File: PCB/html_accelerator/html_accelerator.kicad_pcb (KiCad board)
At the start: 4 copper layers, 129.3 x 104.4 mm, 170 parts, among them J1 Bus_PCI_Express_x16, J2 PCIexpress_bracket, U1 MCS9990, U10 AU6438BS, U11 EMMC_4G, U12 MCS9990, U2 AP1513, U3 CAT24C256YI-GT3, U4 AU6438BS, U5 EMMC_4G, U6 EMMC_4G, U7 EMMC_4G, U8 AU6438BS, U9 AU6438BS, Y1 12MHz, Y2 12MHz, Y3 12MHz, Y4 12MHz, Y5 12MHz

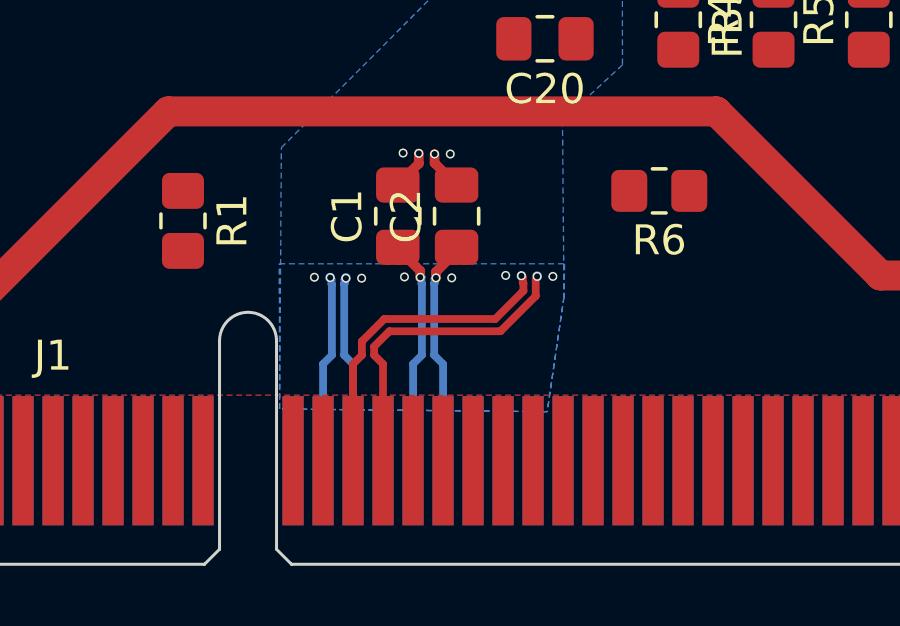
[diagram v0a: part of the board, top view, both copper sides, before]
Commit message: todolist for routing
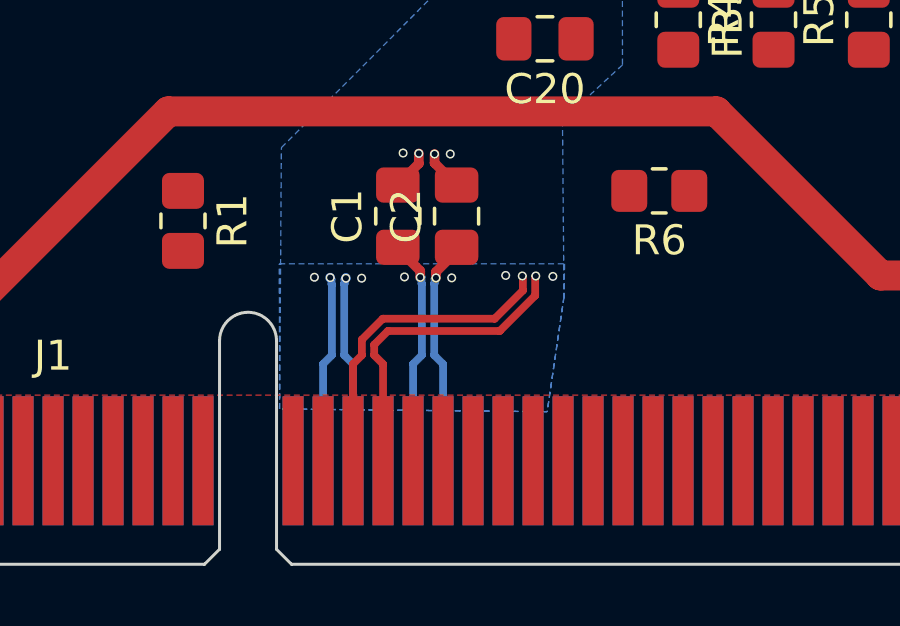
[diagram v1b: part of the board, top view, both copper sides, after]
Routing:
- net /PCIE_Slot/85_PCIE_RX_P: track 44.1 -> 43.1 mm
- net /PCIE_Slot/85_PCIE_RX_N: track 45.2 -> 44.4 mm
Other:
- board text added: "ToDo: update 85 rounting with new cleaner rules"
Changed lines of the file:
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@@
+    (effects (font (size 1.5 1.5) (thickness 0.3) bold) (justify left bottom))
+  )
+  (gr_text "ToDo:\nupdate 85 rounting with new cleaner rules" (at 164.81 151.53) (layer "Eco2.User")
     (effects (font (size 1.5 1.5) (thickness 0.3) bold) (justify left bottom))
   )
@@
   (segment (start 174.983 156.121) (end 174.983 152.895999) (width 0.2593) (layer "B.Cu") (net 746))
   (segment (start 174.68765 152.600649) (end 174.68765 150.226878) (width 0.2593) (layer "B.Cu") (net 746))
-  (segment (start 174.983 156.121) (end 174.983 152.895999) (width 0.2593) (layer "F.Cu") (net 747))
-  (segment (start 179.72523 151.39535) (end 180.663547 150.457033) (width 0.2593) (layer "F.Cu") (net 747))
-  (segment (start 175.27835 152.141991) (end 176.024991 151.39535) (width 0.2593) (layer "F.Cu") (net 747))
+  (segment (start 174.983 152.895999) (end 175.27835 152.600649) (width 0.2593) (layer "F.Cu") (net 747))
+  (segment (start 175.97523 151.38535) (end 179.70523 151.38535) (width 0.2593) (layer "F.Cu") (net 747))
+  (segment (start 179.70523 151.38535) (end 180.64535 150.44523) (width 0.2593) (layer "F.Cu") (net 747))
+  (segment (start 180.64535 150.44523) (end 180.64535 149.98035) (width 0.2593) (layer "F.Cu") (net 747))
   (segment (start 183.945 127.195) (end 183.945 127.860476) (width 0.2507) (layer "F.Cu") (net 747))
-  (segment (start 176.024991 151.39535) (end 179.72523 151.39535) (width 0.2593) (layer "F.Cu") (net 747))
+  (segment (start 175.27835 152.08223) (end 175.97523 151.38535) (width 0.2593) (layer "F.Cu") (net 747))
   (segment (start 183.945 127.860476) (end 183.85965 127.945826) (width 0.2507) (layer "F.Cu") (net 747))
   (segment (start 183.85965 127.945826) (end 183.85965 128.775) (width 0.2507) (layer "F.Cu") (net 747))
-  (segment (start 180.642846 150.001449) (end 180.596397 149.955) (width 0.2507) (layer "F.Cu") (net 747))
-  (segment (start 180.663547 150.196878) (end 180.640347 150.173678) (width 0.2593) (layer "F.Cu") (net 747))
-  (segment (start 180.640347 149.99895) (end 180.596397 149.955) (width 0.2593) (layer "F.Cu") (net 747))
-  (segment (start 180.663547 150.457033) (end 180.663547 150.196878) (width 0.2593) (layer "F.Cu") (net 747))
-  (segment (start 180.640347 150.173678) (end 180.640347 149.99895) (width 0.2593) (layer "F.Cu") (net 747))
+  (segment (start 174.983 156.121) (end 174.983 152.895999) (width 0.2593) (layer "F.Cu") (net 747))
+  (segment (start 180.64535 149.98035) (end 180.625 149.96) (width 0.2593) (layer "F.Cu") (net 747))
   (segment (start 174.983 156.121) (end 174.983 154.321) (width 0.2593) (layer "F.Cu") (net 747))
-  (segment (start 174.983 152.895999) (end 175.27835 152.600649) (width 0.2593) (layer "F.Cu") (net 747))
-  (segment (start 175.27835 152.600649) (end 175.27835 152.141991) (width 0.2593) (layer "F.Cu") (net 747))
+  (segment (start 175.27835 152.600649) (end 175.27835 152.08223) (width 0.2593) (layer "F.Cu") (net 747))
   (via (at 183.945 127.195) (size 0.3) (drill 0.2) (layers "F.Cu" "B.Cu") (net 747))
-  (via (at 180.596397 149.955) (size 0.3) (drill 0.2) (layers "F.Cu" "B.Cu") (free) (net 747))
+  (via (at 180.625 149.96) (size 0.3) (drill 0.2) (layers "F.Cu" "B.Cu") (net 747))
   (segment (start 186.65465 127.142634) (end 186.65465 130.847366) (width 0.2007) (layer "In2.Cu") (net 747))
-  (segment (start 180.596397 149.955) (end 180.622846 149.928551) (width 0.2507) (layer "In2.Cu") (net 747))
   (segment (start 182.74465 132.417366) (end 182.74465 142.037366) (width 0.2007) (layer "In2.Cu") (net 747))
   (segment (start 186.273328 126.761312) (end 186.65465 127.142634) (width 0.2007) (layer "In2.Cu") (net 747))
@@
   (segment (start 183.117366 132.04465) (end 182.74465 132.417366) (width 0.2007) (layer "In2.Cu") (net 747))
   (segment (start 183.945 127.195) (end 183.945 127.002271) (width 0.2007) (layer "In2.Cu") (net 747))
-  (segment (start 180.672847 144.109169) (end 180.672847 149.87855) (width 0.2007) (layer "In2.Cu") (net 747))
-  (segment (start 180.672847 149.87855) (end 180.596397 149.955) (width 0.2007) (layer "In2.Cu") (net 747))
   (segment (start 186.65465 130.847366) (end 185.457366 132.04465) (width 0.2007) (layer "In2.Cu") (net 747))
+  (segment (start 180.625 149.96) (end 180.60535 149.94035) (width 0.2593) (layer "In2.Cu") (net 747))
   (segment (start 184.185959 126.761312) (end 186.273328 126.761312) (width 0.2007) (layer "In2.Cu") (net 747))
+  (segment (start 180.60535 149.94035) (end 180.60535 144.98) (width 0.2593) (layer "In2.Cu") (net 747))
   (segment (start 185.457366 132.04465) (end 183.117366 132.04465) (width 0.2007) (layer "In2.Cu") (net 747))
   (segment (start 183.945 127.002271) (end 184.185959 126.761312) (width 0.2007) (layer "In2.Cu") (net 747))
-  (segment (start 180.596397 149.965) (end 180.596397 149.955) (width 0.3236) (layer "B.Cu") (net 747))
-  (segment (start 175.68765 152.311531) (end 176.194531 151.80465) (width 0.2593) (layer "F.Cu") (net 748))
+  (segment (start 181.05465 149.98035) (end 181.075 149.96) (width 0.2593) (layer "F.Cu") (net 748))
   (segment (start 183.459762 127.945238) (end 183.459762 128.705) (width 0.2507) (layer "F.Cu") (net 748))
+  (segment (start 175.983 156.121) (end 175.983 152.895999) (width 0.2593) (layer "F.Cu") (net 748))
+  (segment (start 181.05465 150.61477) (end 181.05465 149.98035) (width 0.2593) (layer "F.Cu") (net 748))
+  (segment (start 175.68765 152.25177) (end 176.14477 151.79465) (width 0.2593) (layer "F.Cu") (net 748))
+  (segment (start 176.14477 151.79465) (end 179.87477 151.79465) (width 0.2593) (layer "F.Cu") (net 748))
+  (segment (start 179.87477 151.79465) (end 181.05465 150.61477) (width 0.2593) (layer "F.Cu") (net 748))
   (segment (start 175.983 152.895999) (end 175.68765 152.600649) (width 0.2593) (layer "F.Cu") (net 748))
-  (segment (start 176.194531 151.80465) (end 179.89477 151.80465) (width 0.2593) (layer "F.Cu") (net 748))
-  (segment (start 175.68765 152.600649) (end 175.68765 152.311531) (width 0.2593) (layer "F.Cu") (net 748))
-  (segment (start 179.89477 151.80465) (end 181.072847 150.626573) (width 0.2593) (layer "F.Cu") (net 748))
-  (segment (start 181.072847 150.02215) (end 181.119997 149.975) (width 0.2593) (layer "F.Cu") (net 748))
   (segment (start 183.429649 127.021657) (end 183.429649 127.915125) (width 0.2507) (layer "F.Cu") (net 748))
-  (segment (start 181.093548 150.001449) (end 181.119997 149.975) (width 0.2507) (layer "F.Cu") (net 748))
-  (segment (start 175.983 156.121) (end 175.983 152.895999) (width 0.2593) (layer "F.Cu") (net 748))
-  (segment (start 181.072847 150.626573) (end 181.072847 150.02215) (width 0.2593) (layer "F.Cu") (net 748))
   (segment (start 183.429649 127.915125) (end 183.459762 127.945238) (width 0.2507) (layer "F.Cu") (net 748))
   (segment (start 175.983 156.121) (end 175.983 154.321) (width 0.2593) (layer "F.Cu") (net 748))
-  (via (at 181.119997 149.975) (size 0.3) (drill 0.2) (layers "F.Cu" "B.Cu") (free) (net 748))
+  (segment (start 175.68765 152.600649) (end 175.68765 152.25177) (width 0.2593) (layer "F.Cu") (net 748))
+  (via (at 181.075 149.96) (size 0.3) (drill 0.2) (layers "F.Cu" "B.Cu") (net 748))
   (via (at 183.429649 127.021657) (size 0.3) (drill 0.2) (layers "F.Cu" "B.Cu") (net 748))
   (segment (start 183.09535 142.182634) (end 181.023547 144.254437) (width 0.2007) (layer "In2.Cu") (net 748))
-  (segment (start 181.046747 149.90175) (end 181.119997 149.975) (width 0.2007) (layer "In2.Cu") (net 748))
   (segment (start 185.602634 132.39535) (end 183.262634 132.39535) (width 0.2007) (layer "In2.Cu") (net 748))
-  (segment (start 181.023547 144.254437) (end 181.023547 149.745258) (width 0.2007) (layer "In2.Cu") (net 748))
   (segment (start 187.00535 130.992634) (end 185.602634 132.39535) (width 0.2007) (layer "In2.Cu") (net 748))
-  (segment (start 181.046747 149.768458) (end 181.046747 149.90175) (width 0.2007) (layer "In2.Cu") (net 748))
   (segment (start 183.262634 132.39535) (end 183.09535 132.562634) (width 0.2007) (layer "In2.Cu") (net 748))
-  (segment (start 181.119997 149.975) (end 181.073548 149.928551) (width 0.2507) (layer "In2.Cu") (net 748))
+  (segment (start 181.075 149.96) (end 181.09465 149.94035) (width 0.2593) (layer "In2.Cu") (net 748))
   (segment (start 184.040694 126.410612) (end 186.418596 126.410612) (width 0.2007) (layer "In2.Cu") (net 748))
   (segment (start 183.429649 127.021657) (end 184.040694 126.410612) (width 0.2007) (layer "In2.Cu") (net 748))
   (segment (start 187.00535 126.997366) (end 187.00535 130.992634) (width 0.2007) (layer "In2.Cu") (net 748))
-  (segment (start 181.023547 149.745258) (end 181.046747 149.768458) (width 0.2007) (layer "In2.Cu") (net 748))
+  (segment (start 181.09465 149.94035) (end 181.09465 144.98) (width 0.2593) (layer "In2.Cu") (net 748))
   (segment (start 186.418596 126.410612) (end 187.00535 126.997366) (width 0.2007) (layer "In2.Cu") (net 748))
   (segment (start 183.09535 132.562634) (end 183.09535 142.182634) (width 0.2007) (layer "In2.Cu") (net 748))
-  (segment (start 181.119997 149.965) (end 181.119997 149.975) (width 0.3236) (layer "B.Cu") (net 748))
   (segment (start 186.46 132.7625) (end 186.46 132.53) (width 0.25) (layer "F.Cu") (net 751))
   (segment (start 147.7237 132.3237) (end 147.725 132.325) (width 0.2) (layer "F.Cu") (net 754))
